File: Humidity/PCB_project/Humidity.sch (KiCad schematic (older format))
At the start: 11 parts, among them J1 Signals, J2 Power, U1 74HC595

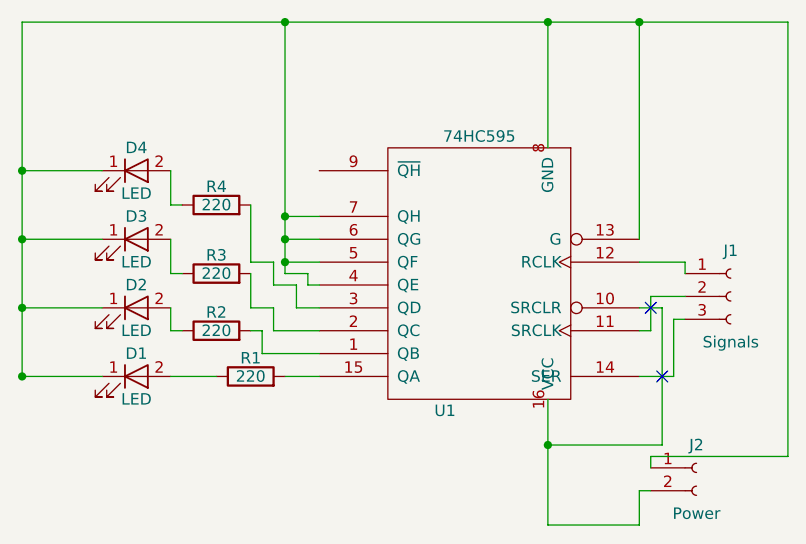
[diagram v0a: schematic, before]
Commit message: PCB for led
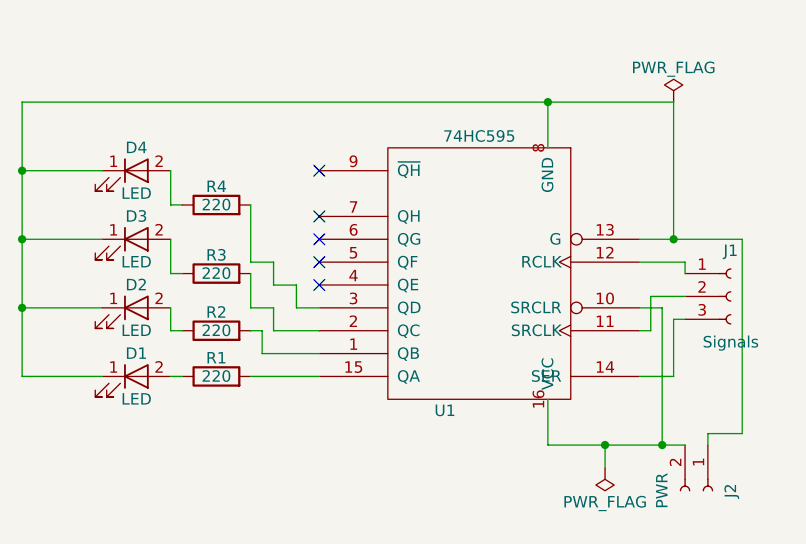
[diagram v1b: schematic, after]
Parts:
- D1, D2, D3, D4: footprint (none) -> LEDs:LED-5MM
- J1: footprint (none) -> Socket_Strips:Socket_Strip_Straight_1x03_Pitch2.54mm
- J2: value Power -> PWR; footprint (none) -> Socket_Strips:Socket_Strip_Straight_1x02_Pitch2.54mm
- R1, R2, R3, R4: footprint (none) -> Resistors_THT:R_Axial_DIN0207_L6.3mm_D2.5mm_P2.54mm_Vertical
- U1: footprint (none) -> Housings_DIP:DIP-16_W7.62mm
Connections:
- net at D1.1 (K), D2.1 (K), D3.1 (K)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: no longer U1.4 (QE), U1.5 (QF), U1.6 (QG), U1.7 (QH)
- no-connect marks 2 -> 5
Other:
- moved on the sheet: R1
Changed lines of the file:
@@
 F 0 "U1" H 5250 3950 50  0000 C CNN
 F 1 "74HC595" H 5100 2750 50  0000 C CNN
-F 2 "" H 5100 3350 50  0001 C CNN
+F 2 "Housings_DIP:DIP-16_W7.62mm" H 5100 3350 50  0001 C CNN
 F 3 "" H 5100 3350 50  0001 C CNN
 	1    5100 3350
@@
 F 0 "D4" H 3600 3000 50  0000 C CNN
 F 1 "LED" H 3600 2800 50  0000 C CNN
-F 2 "" H 3600 2900 50  0001 C CNN
+F 2 "LEDs:LED-5MM" H 3600 2900 50  0001 C CNN
 F 3 "" H 3600 2900 50  0001 C CNN
 	1    3600 2900
@@
 F 0 "D3" H 3600 3300 50  0000 C CNN
 F 1 "LED" H 3600 3100 50  0000 C CNN
-F 2 "" H 3600 3200 50  0001 C CNN
+F 2 "LEDs:LED-5MM" H 3600 3200 50  0001 C CNN
 F 3 "" H 3600 3200 50  0001 C CNN
 	1    3600 3200
@@
 F 0 "D2" H 3600 3600 50  0000 C CNN
 F 1 "LED" H 3600 3400 50  0000 C CNN
-F 2 "" H 3600 3500 50  0001 C CNN
+F 2 "LEDs:LED-5MM" H 3600 3500 50  0001 C CNN
 F 3 "" H 3600 3500 50  0001 C CNN
 	1    3600 3500
@@
 F 0 "D1" H 3600 3900 50  0000 C CNN
 F 1 "LED" H 3600 3700 50  0000 C CNN
-F 2 "" H 3600 3800 50  0001 C CNN
+F 2 "LEDs:LED-5MM" H 3600 3800 50  0001 C CNN
 F 3 "" H 3600 3800 50  0001 C CNN
 	1    3600 3800
@@
 F 0 "R4" V 4030 3050 50  0000 C CNN
 F 1 "220" V 3950 3050 50  0000 C CNN
-F 2 "" V 3880 3050 50  0001 C CNN
+F 2 "Resistors_THT:R_Axial_DIN0207_L6.3mm_D2.5mm_P2.54mm_Vertical" V 3880 3050 50  0001 C CNN
 F 3 "" H 3950 3050 50  0001 C CNN
 	1    3950 3050
@@
 F 0 "R3" V 4030 3350 50  0000 C CNN
 F 1 "220" V 3950 3350 50  0000 C CNN
-F 2 "" V 3880 3350 50  0001 C CNN
+F 2 "Resistors_THT:R_Axial_DIN0207_L6.3mm_D2.5mm_P2.54mm_Vertical" V 3880 3350 50  0001 C CNN
 F 3 "" H 3950 3350 50  0001 C CNN
 	1    3950 3350
@@
 F 0 "R2" V 4030 3600 50  0000 C CNN
 F 1 "220" V 3950 3600 50  0000 C CNN
-F 2 "" V 3880 3600 50  0001 C CNN
+F 2 "Resistors_THT:R_Axial_DIN0207_L6.3mm_D2.5mm_P2.54mm_Vertical" V 3880 3600 50  0001 C CNN
 F 3 "" H 3950 3600 50  0001 C CNN
 	1    3950 3600
@@
 L R R1
 U 1 1 5ABC1588
-P 4100 3800
-F 0 "R1" V 4180 3800 50  0000 C CNN
-F 1 "220" V 4100 3800 50  0000 C CNN
-F 2 "" V 4030 3800 50  0001 C CNN
-F 3 "" H 4100 3800 50  0001 C CNN
-	1    4100 3800
-	0    -1   -1   0
-$EndComp
-Wire Wire Line
-	4250 3800 4400 3800
-Wire Wire Line
-	3750 3800 3950 3800
+P 3950 3800
+F 0 "R1" V 4030 3800 50  0000 C CNN
+F 1 "220" V 3950 3800 50  0000 C CNN
+F 2 "Resistors_THT:R_Axial_DIN0207_L6.3mm_D2.5mm_P2.54mm_Vertical" V 3880 3800 50  0001 C CNN
+F 3 "" H 3950 3800 50  0001 C CNN
+	1    3950 3800
+	0    -1   -1   0
+$EndComp
+Wire Wire Line
+	4100 3800 4400 3800
+Wire Wire Line
+	3750 3800 3800 3800
 Wire Wire Line
 	3750 2900 3750 3050
@@
 	4300 3500 4400 3500
 Wire Wire Line
-	3450 2900 3100 2900
-Wire Wire Line
 	3100 3200 3450 3200
-Connection ~ 3100 3200
 Wire Wire Line
 	3100 3500 3450 3500
-Connection ~ 3100 3500
 Wire Wire Line
 	3100 3800 3450 3800
-Connection ~ 3100 3800
-Wire Wire Line
-	3100 2250 6450 2250
-Connection ~ 3100 2900
-Wire Wire Line
-	3100 2250 3100 3800
-Wire Wire Line
-	5800 2250 5800 3200
-Connection ~ 5400 2250
-Wire Wire Line
-	5400 4450 5800 4450
-$Comp
-L Conn_01x02_Female J2
-U 1 1 5ABC29BA
-P 6050 4200
-F 0 "J2" H 6050 4300 50  0000 C CNN
-F 1 "Power" H 6050 4000 50  0000 C CNN
-F 2 "" H 6050 4200 50  0001 C CNN
-F 3 "" H 6050 4200 50  0001 C CNN
-	1    6050 4200
-	1    0    0    -1
-$EndComp
 $Comp
 L Conn_01x03_Female J1
@@
 F 0 "J1" H 6200 3650 50  0000 C CNN
 F 1 "Signals" H 6200 3250 50  0000 C CNN
-F 2 "" H 6200 3450 50  0001 C CNN
+F 2 "Socket_Strips:Socket_Strip_Straight_1x03_Pitch2.54mm" H 6200 3450 50  0001 C CNN
 F 3 "" H 6200 3450 50  0001 C CNN
 	1    6200 3450
@@
 	6000 3300 6000 3350
 Wire Wire Line
+	5800 3600 5850 3600
+Wire Wire Line
+	5850 3600 5850 3450
+Wire Wire Line
+	5850 3450 6000 3450
+Wire Wire Line
+	5800 3800 5950 3800
+Wire Wire Line
+	5950 3800 5950 3550
+Wire Wire Line
+	5950 3550 6000 3550
+NoConn ~ 4400 2900
+NoConn ~ 4400 3100
+NoConn ~ 4400 3200
+NoConn ~ 4400 3300
+NoConn ~ 4400 3400
+Wire Wire Line
+	5800 3200 6250 3200
+Wire Wire Line
+	3450 2900 3100 2900
+Wire Wire Line
+	5400 3900 5400 4100
+Wire Wire Line
 	5800 3500 5900 3500
 Wire Wire Line
+	3100 3800 3100 2600
+Wire Wire Line
+	3100 2600 5950 2600
+Wire Wire Line
+	5950 2600 5950 3200
+$Comp
+L PWR_FLAG #FLG01
+U 1 1 5ABD5AF7
+P 5950 2600
+F 0 "#FLG01" H 5950 2675 50  0001 C CNN
+F 1 "PWR_FLAG" H 5950 2750 50  0000 C CNN
+F 2 "" H 5950 2600 50  0001 C CNN
+F 3 "" H 5950 2600 50  0001 C CNN
+	1    5950 2600
+	1    0    0    -1
+$EndComp
+$Comp
+L PWR_FLAG #FLG02
+U 1 1 5ABD5B65
+P 5650 4200
+F 0 "#FLG02" H 5650 4275 50  0001 C CNN
+F 1 "PWR_FLAG" H 5650 4350 50  0000 C CNN
+F 2 "" H 5650 4200 50  0001 C CNN
+F 3 "" H 5650 4200 50  0001 C CNN
+	1    5650 4200
+	-1   0    0    1
+$EndComp
+Connection ~ 5400 2600
+Connection ~ 3100 2900
+Connection ~ 3100 3200
+Connection ~ 3100 3500
+$Comp
+L Conn_01x02_Female J2
+U 1 1 5ABD5D68
+P 6100 4300
+F 0 "J2" H 6100 4400 50  0000 C CNN
+F 1 "PWR" H 6100 4100 50  0000 C CNN
+F 2 "Socket_Strips:Socket_Strip_Straight_1x02_Pitch2.54mm" H 6100 4300 50  0001 C CNN
+F 3 "" H 6100 4300 50  0001 C CNN
+	1    6100 4300
+	0    1    1    0
+$EndComp
+Wire Wire Line
+	5400 4100 6000 4100
+Wire Wire Line
+	5650 4200 5650 4100
+Connection ~ 5650 4100
+Wire Wire Line
 	5900 3500 5900 4100
-Wire Wire Line
-	5800 4450 5800 4300
-Wire Wire Line
-	5800 4300 5850 4300
-Wire Wire Line
-	5800 3600 5850 3600
-Wire Wire Line
-	5850 3600 5850 3450
-Wire Wire Line
-	5850 3450 6000 3450
-Wire Wire Line
-	5800 3800 5950 3800
-Wire Wire Line
-	5950 3800 5950 3550
-Wire Wire Line
-	5950 3550 6000 3550
-NoConn ~ 5850 3500
-NoConn ~ 5900 3800
-Wire Wire Line
-	5400 2800 5400 2250
-Wire Wire Line
-	5400 3900 5400 4450
-Wire Wire Line
-	4400 3400 4350 3400
-Wire Wire Line
-	4350 3400 4350 3350
-Wire Wire Line
-	4350 3350 4250 3350
-Wire Wire Line
-	4250 3350 4250 2250
-Connection ~ 4250 2250
-Wire Wire Line
-	4400 3300 4250 3300
-Connection ~ 4250 3300
-Wire Wire Line
-	4400 3200 4250 3200
-Connection ~ 4250 3200
-Wire Wire Line
-	4400 3100 4250 3100
-Connection ~ 4250 3100
-Wire Wire Line
-	5900 4100 5400 4100
-Connection ~ 5400 4100
-Wire Wire Line
-	5850 4200 5850 4150
-Wire Wire Line
-	5850 4150 6450 4150
-Wire Wire Line
-	6450 4150 6450 2250
-Connection ~ 5800 2250
+Connection ~ 5900 4100
+Wire Wire Line
+	6250 3200 6250 4050
+Wire Wire Line
+	6250 4050 6100 4050
+Wire Wire Line
+	6100 4050 6100 4100
+Connection ~ 5950 3200
+Wire Wire Line
+	5400 2800 5400 2600
 $EndSCHEMATC
